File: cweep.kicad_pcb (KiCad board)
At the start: 2 copper layers, 107.6 x 84 mm, 39 parts, among them SW1 SW_Push, SW10 SW_Push, SW11 SW_Push, SW12 SW_Push, SW13 SW_Push, SW14 SW_Push, SW15 SW_Push, SW16 SW_Push, SW17 SW_Push, SW2 SW_Push, SW3 SW_Push, SW4 SW_Push, SW5 SW_Push, SW6 SW_Push, SW7 SW_Push, SW8 SW_Push, SW9 SW_Push, U1 XIAO-nRF52840, U2 BQ25504RGTR

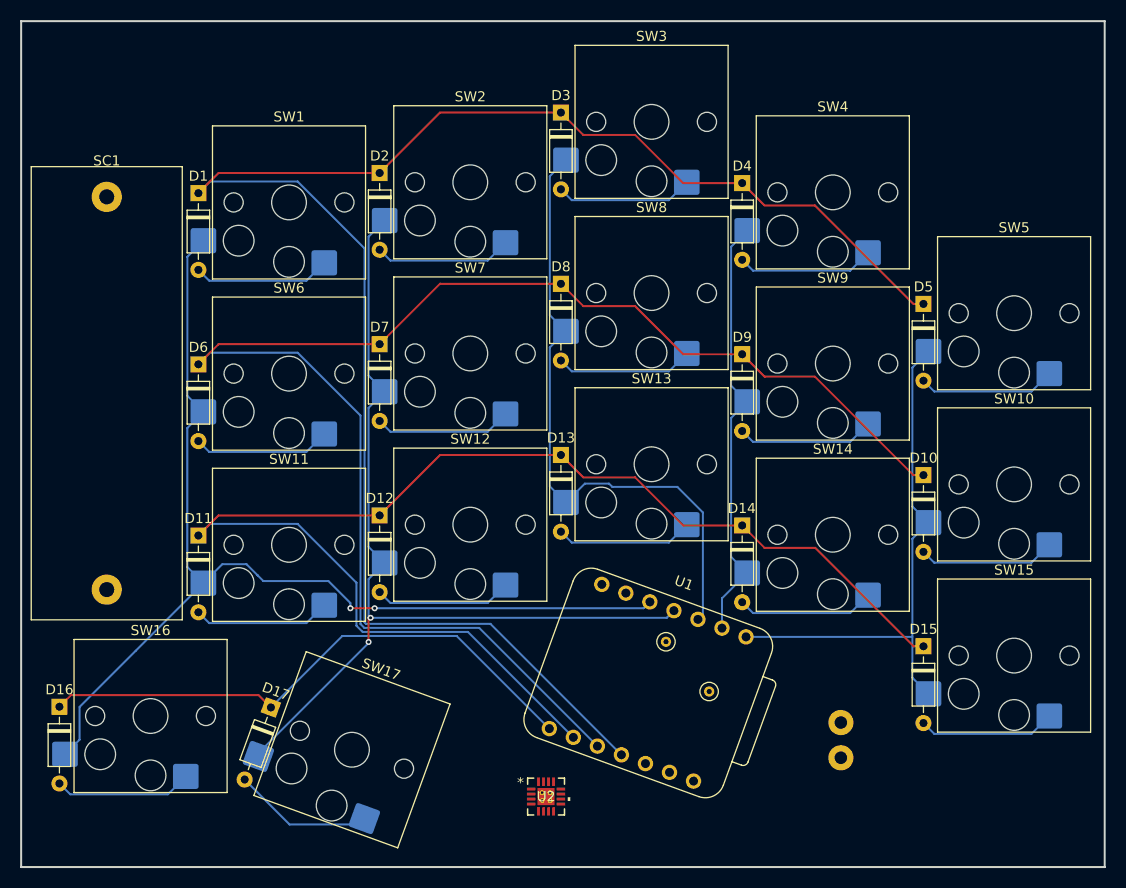
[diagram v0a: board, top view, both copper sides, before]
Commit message: feat: add battery
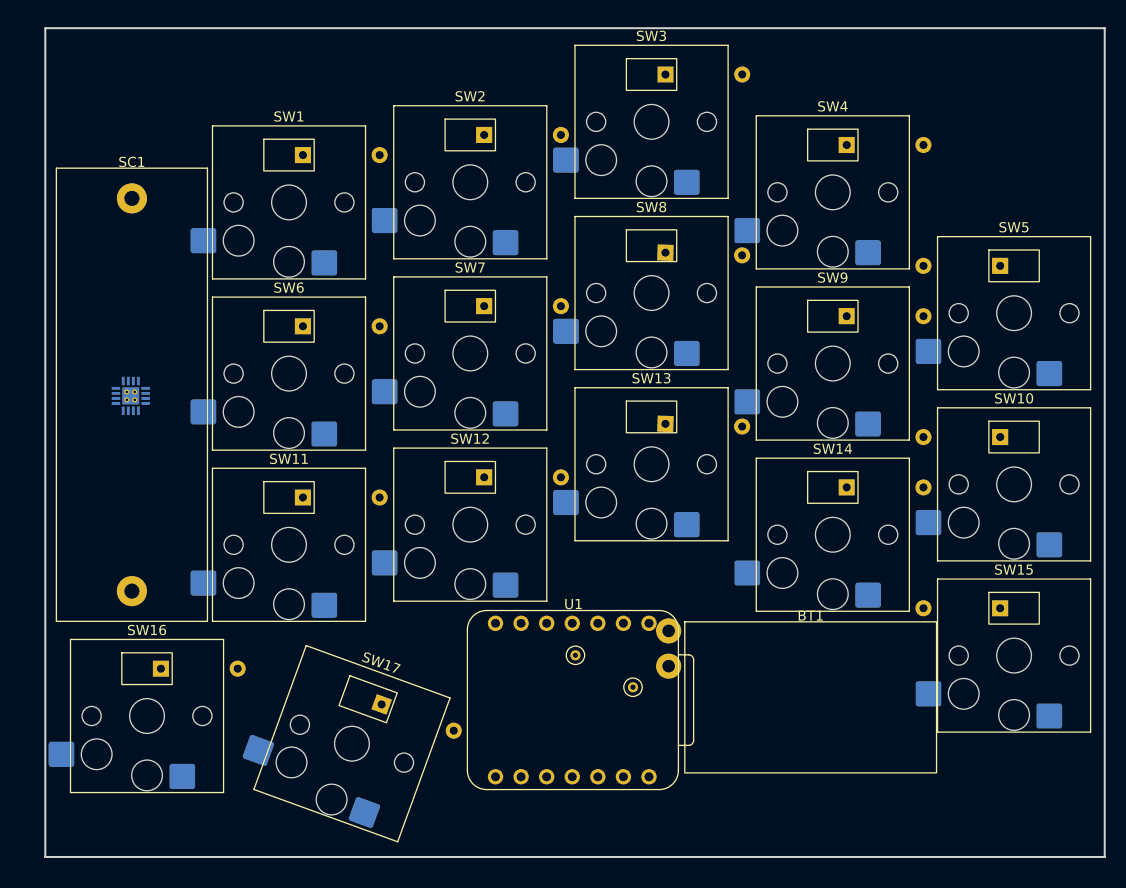
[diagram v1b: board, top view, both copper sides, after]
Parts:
- removed BAT+1, BAT-1: MountingHole_Pad, TOTEM:BatteryPad
- added BT1: 3.7V LiPo, cweep:battery-13853-sparkfun-25x15x4, F.Cu at (238.8, 100.2)
- D1, D10, D11, D12, D13, D14, D15, D16, D17, D2, D3, D4, D5, D6, D7, D8, D9: footprint cweep:D_DO-35_SOD27_P7.62mm_Horizontal -> Diode_THT:D_DO-35_SOD27_P7.62mm_Horizontal; moved to B.Cu
- U2: moved to B.Cu
- moved U2 57.3 mm to (171.3, 70.2), turned to 180 degrees
- moved D17 15.8 mm to (196.2, 100.8)
- moved D1 15.7 mm to (188.4, 46.3)
- moved D11 15.7 mm to (188.4, 80.3)
- moved D12 15.7 mm to (206.4, 78.3)
- moved D14 15.7 mm to (242.4, 79.3)
- moved D2 15.7 mm to (206.4, 44.3)
- moved D3 15.7 mm to (224.4, 38.3)
- moved D4 15.7 mm to (242.4, 45.3)
- moved D6 15.7 mm to (188.4, 63.3)
- moved D7 15.7 mm to (206.4, 61.3)
- moved D9 15.7 mm to (242.4, 62.3)
- moved D16 15.5 mm to (174.3, 97.3)
- moved D13 15.2 mm to (224.4, 73.0), turned to -2 degrees
- moved D8 15.2 mm to (224.4, 56.0), turned to -2 degrees
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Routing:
- net /row 0: track 171.0 -> 0.00 mm
- net /row 1: track 151.6 -> 0.00 mm
- net /row 2: track 132.2 -> 0.00 mm
- net /column 0: track 106.8 -> 0.00 mm, vias 2 -> 0
- net /column 1: track 91.9 -> 0.00 mm, vias 2 -> 0
- net /column 2: track 63.0 -> 0.00 mm
- net /row 3: track 56.4 -> 0.00 mm
- net /column 4: track 53.2 -> 0.00 mm
- net /column 3: track 43.2 -> 0.00 mm
- net Net-(D17-A): track 14.0 -> 0.00 mm
- net Net-(D16-A): track 13.7 -> 0.00 mm
- net Net-(D4-A): track 13.7 -> 0.00 mm
- net Net-(D3-A): track 13.7 -> 0.00 mm
- net Net-(D2-A): track 13.7 -> 0.00 mm
- net Net-(D1-A): track 13.7 -> 0.00 mm
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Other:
- board size 107.6 x 84 mm -> 105.2 x 82.3 mm
- board text added: "put reset button here"
